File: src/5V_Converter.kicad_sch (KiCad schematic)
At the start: 13 parts, among them U3 TPS564257DRLR (12V-5V)

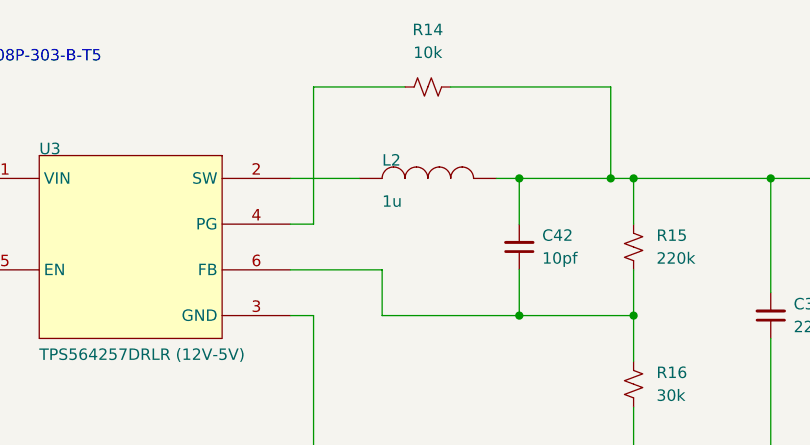
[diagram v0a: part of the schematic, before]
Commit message: Pushing remaining schematic files
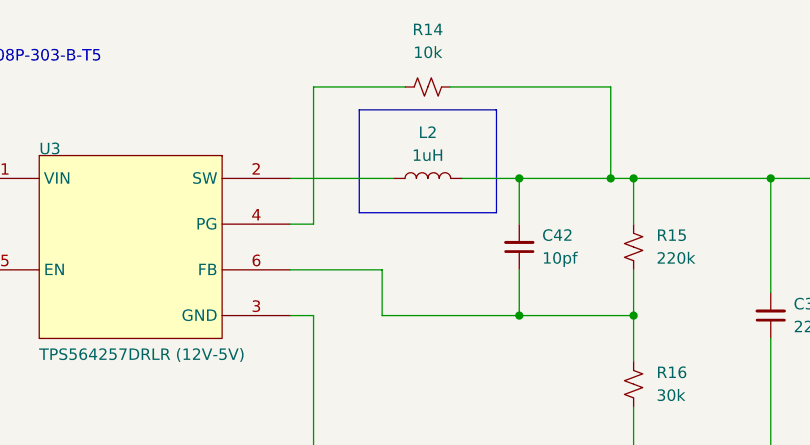
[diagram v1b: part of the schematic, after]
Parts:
- removed L2: Inductor, symbol Simulation Generic Components:Inductor
- added L2: 1uH, symbol Device:L
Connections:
- net Vout+: now also L2.2
- net at U3.2 (SW): now also L2.1
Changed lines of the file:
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@@
 	(generator_version "10.0")
 	(paper "A")
+	(rectangle
+		(start 127 83.82)
+		(end 142.24 95.25)
+		(stroke
+			(width 0)
+			(type solid)
+			(color 255 7 0 1)
+		)
+		(fill
+			(type none)
+		)
+	)
 	(text "Susumu Co LtdRG1608P-303-B-T5"
 		(exclude_from_sim no)
@@
 	(wire
 		(pts
-			(xy 127 91.44) (xy 119.38 91.44)
+			(xy 119.38 91.44) (xy 130.81 91.44)
 		)
 		(stroke
@@
 	(wire
 		(pts
-			(xy 144.78 91.44) (xy 142.24 91.44)
-		)
-		(stroke
-			(width 0)
-			(type default)
-		)
-	)
-	(wire
-		(pts
 			(xy 154.94 91.44) (xy 144.78 91.44)
 		)
@@
 		(pts
 			(xy 144.78 96.52) (xy 144.78 91.44)
+		)
+		(stroke
+			(width 0)
+			(type default)
+		)
+	)
+	(wire
+		(pts
+			(xy 138.43 91.44) (xy 144.78 91.44)
 		)
 		(stroke
@@
 	)
 	(symbol
-		(lib_id "Simulation Generic Components:Inductor")
-		(at 127 91.44 0)
+		(lib_id "Device:L")
+		(at 134.62 91.44 90)
 		(unit 1)
 		(body_style 1)
@@
 		(in_pos_files yes)
 		(dnp no)
+		(fields_autoplaced yes)
 		(property "Reference" "L2"
-			(at 129.54 90.17 0)
-			(show_name no)
-			(do_not_autoplace no)
-			(effects
-				(font
-					(size 1.27 1.27)
-				)
-				(justify left bottom)
-			)
-		)
-		(property "Value" "Inductor"
-			(at 129.54 94.742 0)
-			(hide yes)
-			(show_name no)
-			(do_not_autoplace no)
-			(effects
-				(font
-					(size 1.27 1.27)
-				)
-				(justify left bottom)
+			(at 134.62 86.36 90)
+			(show_name no)
+			(do_not_autoplace no)
+			(effects
+				(font
+					(size 1.27 1.27)
+				)
+			)
+		)
+		(property "Value" "1uH"
+			(at 134.62 88.9 90)
+			(show_name no)
+			(do_not_autoplace no)
+			(effects
+				(font
+					(size 1.27 1.27)
+				)
 			)
 		)
 		(property "Footprint" ""
-			(at 127 91.44 0)
+			(at 134.62 91.44 0)
 			(hide yes)
 			(show_name no)
@@
 		)
 		(property "Datasheet" ""
-			(at 127 91.44 0)
+			(at 134.62 91.44 0)
 			(hide yes)
 			(show_name no)
@@
 		)
 		(property "Description" "Inductor"
-			(at 127 91.44 0)
-			(hide yes)
-			(show_name no)
-			(do_not_autoplace no)
-			(effects
-				(font
-					(size 1.27 1.27)
-				)
-			)
-		)
-		(property "SIMULATIONGENERICCOMPONENT" "True"
-			(at 129.54 97.282 0)
-			(hide yes)
-			(show_name no)
-			(do_not_autoplace no)
-			(effects
-				(font
-					(size 1.27 1.27)
-				)
-				(justify left bottom)
-			)
-		)
-		(property "DTEMP" ""
-			(at 142.748 92.202 0)
-			(hide yes)
-			(show_name no)
-			(do_not_autoplace no)
-			(effects
-				(font
-					(size 1.27 1.27)
-				)
-				(justify left bottom)
-			)
-		)
-		(property "T_REL_LOCAL" ""
-			(at 142.748 92.202 0)
-			(hide yes)
-			(show_name no)
-			(do_not_autoplace no)
-			(effects
-				(font
-					(size 1.27 1.27)
-				)
-				(justify left bottom)
-			)
-		)
-		(property "INITIAL CURRENT" ""
-			(at 142.748 92.202 0)
-			(hide yes)
-			(show_name no)
-			(do_not_autoplace no)
-			(effects
-				(font
-					(size 1.27 1.27)
-				)
-				(justify left bottom)
-			)
-		)
-		(property "CPAR" ""
-			(at 142.748 92.202 0)
-			(hide yes)
-			(show_name no)
-			(do_not_autoplace no)
-			(effects
-				(font
-					(size 1.27 1.27)
-				)
-				(justify left bottom)
-			)
-		)
-		(property "M" ""
-			(at 142.748 92.202 0)
-			(hide yes)
-			(show_name no)
-			(do_not_autoplace no)
-			(effects
-				(font
-					(size 1.27 1.27)
-				)
-				(justify left bottom)
-			)
-		)
-		(property "RPAR" ""
-			(at 142.748 92.202 0)
-			(hide yes)
-			(show_name no)
-			(do_not_autoplace no)
-			(effects
-				(font
-					(size 1.27 1.27)
-				)
-				(justify left bottom)
-			)
-		)
-		(property "RSER" ""
-			(at 142.748 92.202 0)
-			(hide yes)
-			(show_name no)
-			(do_not_autoplace no)
-			(effects
-				(font
-					(size 1.27 1.27)
-				)
-				(justify left bottom)
-			)
-		)
-		(property "TC1" ""
-			(at 142.748 92.202 0)
-			(hide yes)
-			(show_name no)
-			(do_not_autoplace no)
-			(effects
-				(font
-					(size 1.27 1.27)
-				)
-				(justify left bottom)
-			)
-		)
-		(property "TC2" ""
-			(at 142.748 92.202 0)
-			(hide yes)
-			(show_name no)
-			(do_not_autoplace no)
-			(effects
-				(font
-					(size 1.27 1.27)
-				)
-				(justify left bottom)
-			)
-		)
-		(property "TEMP" ""
-			(at 142.748 92.202 0)
-			(hide yes)
-			(show_name no)
-			(do_not_autoplace no)
-			(effects
-				(font
-					(size 1.27 1.27)
-				)
-				(justify left bottom)
-			)
-		)
-		(property "ALTIUM_VALUE" "1u"
-			(at 129.54 94.742 0)
-			(show_name no)
-			(do_not_autoplace no)
-			(effects
-				(font
-					(size 1.27 1.27)
-				)
-				(justify left bottom)
-			)
+			(at 134.62 91.44 0)
+			(hide yes)
+			(show_name no)
+			(do_not_autoplace no)
+			(effects
+				(font
+					(size 1.27 1.27)
+				)
+			)
+		)
+		(pin "2"
 		)
 		(pin "1"
 		)
-		(pin "2"
-		)
 		(instances
